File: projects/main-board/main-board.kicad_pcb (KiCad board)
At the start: 4 copper layers, 165 x 68 mm, 211 parts, among them J1 TC2030, J2 TC2030, J3 S3B-PH-SM4-TB, J4 USB4105-GF-A, J5 TC2030, J6 NHD-4.3-480272EF-ASXP (Molex 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, J7 USB4105-GF-A, Q1 ZXTN4240F-7, Q2 ZXTN4240F-7, SW1 450404015514, SW10 TS06-667-25-BK-160-G-SMT-TR, SW11 TS06-667-25-BK-160-G-SMT-TR, SW12 TS06-667-25-BK-160-G-SMT-TR, SW13 TS06-667-25-BK-160-G-SMT-TR, SW14 TS06-667-25-BK-160-G-SMT-TR, SW18 TS06-667-25-BK-160-G-SMT-TR, SW2 TS06-667-25-BK-160-G-SMT-TR, SW3 TS06-667-25-BK-160-G-SMT-TR, SW4 TS06-667-25-BK-160-G-SMT-TR, SW5 TS06-667-25-BK-160-G-SMT-TR, SW6 TS06-667-25-BK-160-G-SMT-TR, SW9 TS06-667-25-BK-160-G-SMT-TR, U1 STM32N657X0HxQ, U10 AP5725WG-7, U11 NAU8325YG, U12 TLV74330PDBVR, U13 DM3AT-SF-PEJM5, U14 LSM6DSO32TR, U2 APS256XXN-OBR-BG, U3 MX25UM25645GXDI00, U4 TPS22992RXPR, U5 MPM3805GQB-18-Z, U6 TPSM863253RDXR, U7 MAX77972EWX+T, U8 TS3USB221ARSER, U9 ESP32-C6FH4, Y1 ABM10W-40.0000MHZ-8-B1U-T3

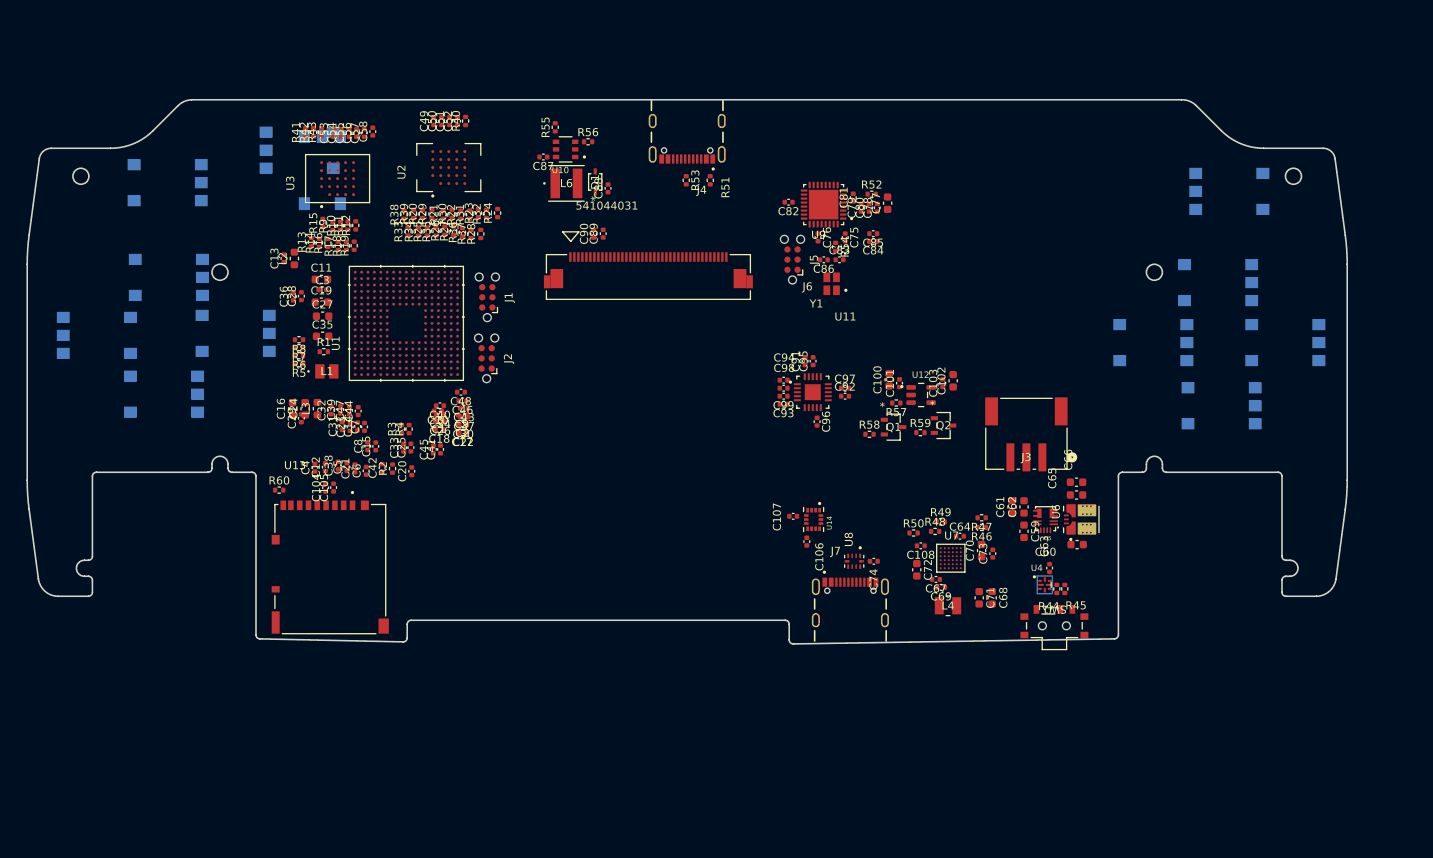
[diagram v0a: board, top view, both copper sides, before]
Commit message: Update render
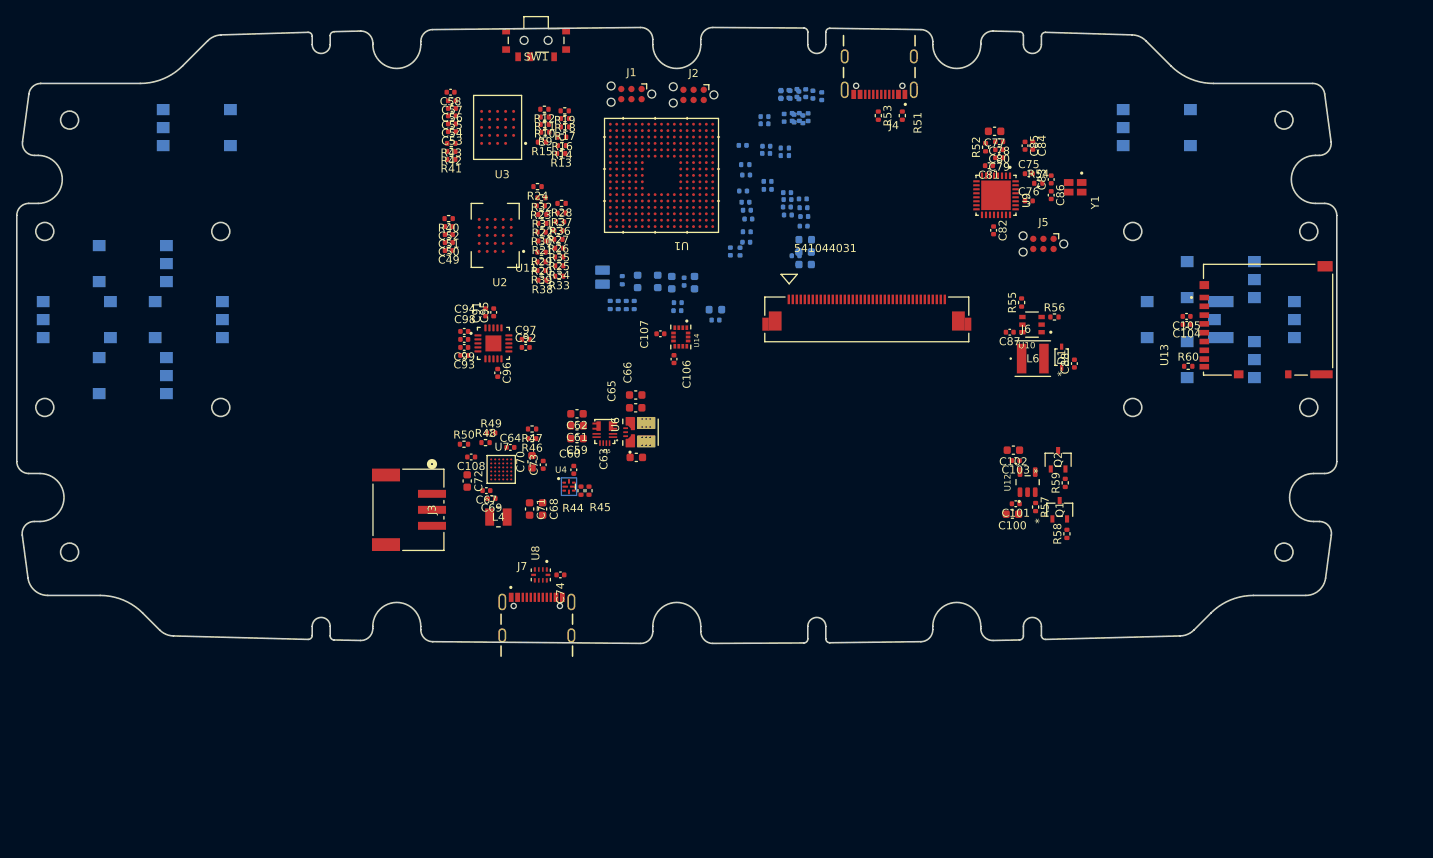
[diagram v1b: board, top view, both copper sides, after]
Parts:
- removed SW13, SW14: TS06-667-25-BK-160-G-SMT-TR, footprint-library:TS06-667-25-BK-160-G-SMT-TR
- C1, C10, C11, C12, C13, C14, C15, C16, C17, C18, C19, C2, C20, C21, C22, C23, C24, C25, C26, C27, C28, C29, C3, C30, C31, C32, C33, C34, C35, C36, C37, C38, C39, C4, C40, C41, C42, C43, C44, C45, C46, C47, C48, C5, C6, C7, C8, C89, C9, C90, L1, L2, L3, R1, R2, R3, R4, R5, R6, R7, R8: moved to B.Cu
- moved U13 121.3 mm to (220.4, 74.8), turned to 90 degrees
- moved R60 114.7 mm to (210.4, 80.7)
- moved C104 109.6 mm to (210.2, 75.4), turned to 180 degrees
- moved C105 108.7 mm to (210.2, 74.4), turned to 180 degrees
- moved SW1 97.7 mm to (128.9, 39.9), turned to 0 degrees
- moved J3 77.8 mm to (113.0, 98.6), turned to 90 degrees
- moved C16 66.6 mm to (162.5, 67.9), turned to 0 degrees
- moved C24 65.5 mm to (162.5, 66.4), turned to 0 degrees
- moved C29 65.0 mm to (161.4, 66.9), turned to 0 degrees
- moved L3 64.5 mm to (162.6, 64.8), turned to 0 degrees
- moved C32 63.4 mm to (162.4, 63.1), turned to 0 degrees
- moved C39 62.8 mm to (162.4, 61.9), turned to 0 degrees
- moved C87 62.3 mm to (188.1, 76.4)
- moved C88 62.3 mm to (196.2, 80.3)
- moved D1 62.3 mm to (194.6, 79.5)
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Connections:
- U1 pad L4: /Buttons/BUTTONS.B10 -> unconnected-(U1F-PF10-PadL4)
- U1 pad P3: /Buttons/BUTTONS.B11 -> unconnected-(U1F-PF11-PadP3)
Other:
- board size 165 x 68 mm -> 165 x 77 mm

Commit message: Update PCB profile and render
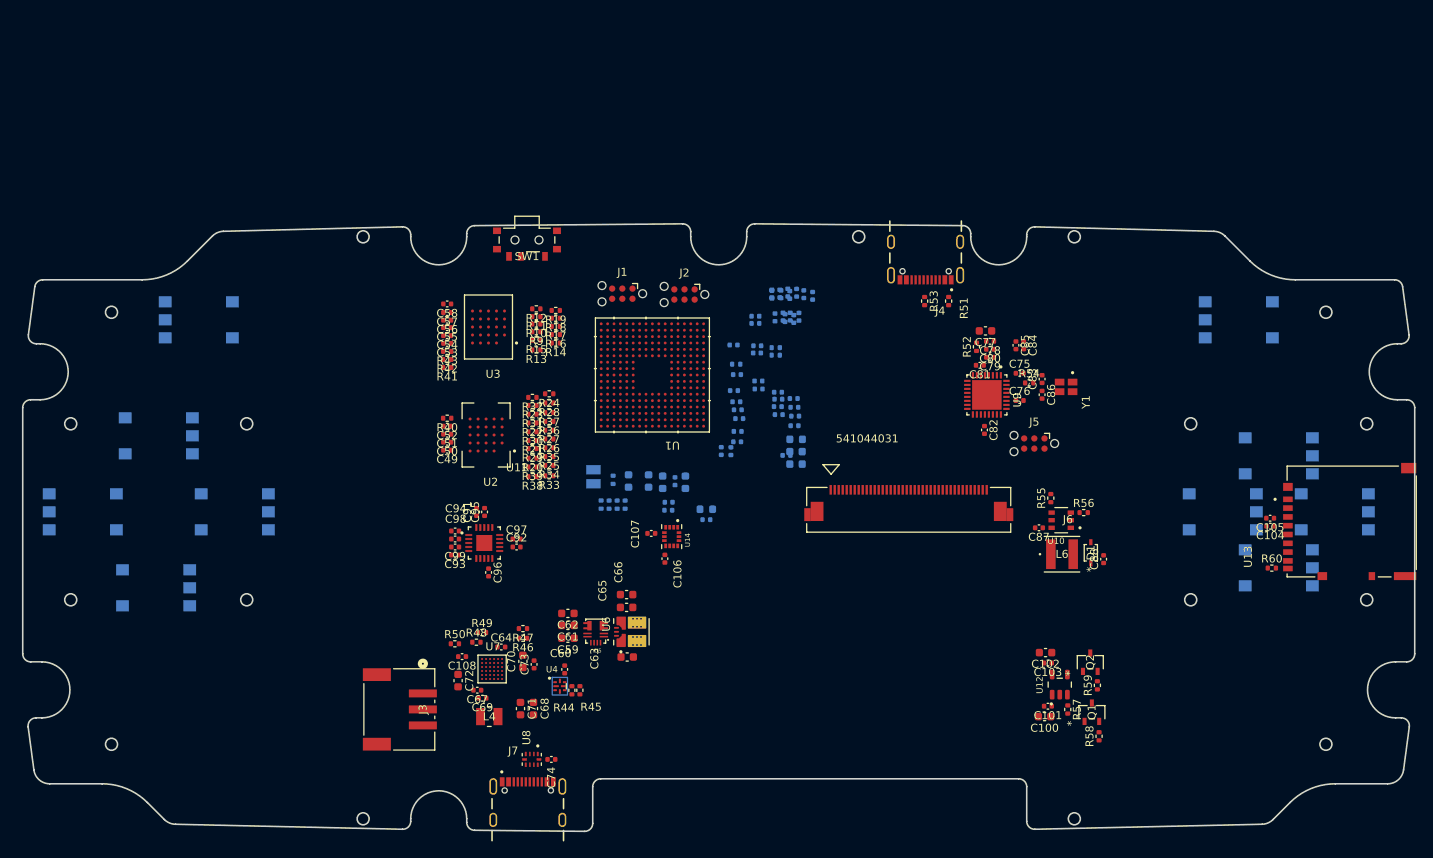
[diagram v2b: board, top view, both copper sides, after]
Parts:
- moved C105 27.3 mm to (220.7, 99.7)
- moved R60 27.3 mm to (220.9, 105.9)
- moved U13 27.3 mm to (230.9, 100.1)
- moved C104 27.3 mm to (220.7, 100.6)
- moved SW9 27.0 mm to (221.8, 105.8)
- moved SW10 26.7 mm to (81.4, 108.3)
- moved C53 26.5 mm to (117.8, 77.8)
- moved C55 26.5 mm to (117.8, 75.8)
- moved C56 26.5 mm to (117.8, 74.9)
- moved C54 26.5 mm to (117.8, 76.8)
- moved C57 26.5 mm to (117.8, 73.9)
- moved C58 26.5 mm to (117.8, 72.9)
- moved SW12 26.1 mm to (216.8, 74.8)
- moved R41 26.0 mm to (117.8, 80.8)
- moved R42 26.0 mm to (117.8, 79.8)
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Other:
- board size 165 x 77 mm -> 174 x 75.9 mm
